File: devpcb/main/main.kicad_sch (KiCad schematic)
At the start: 17 parts, among them U1 DRV8301DCAR, U2 RP2040

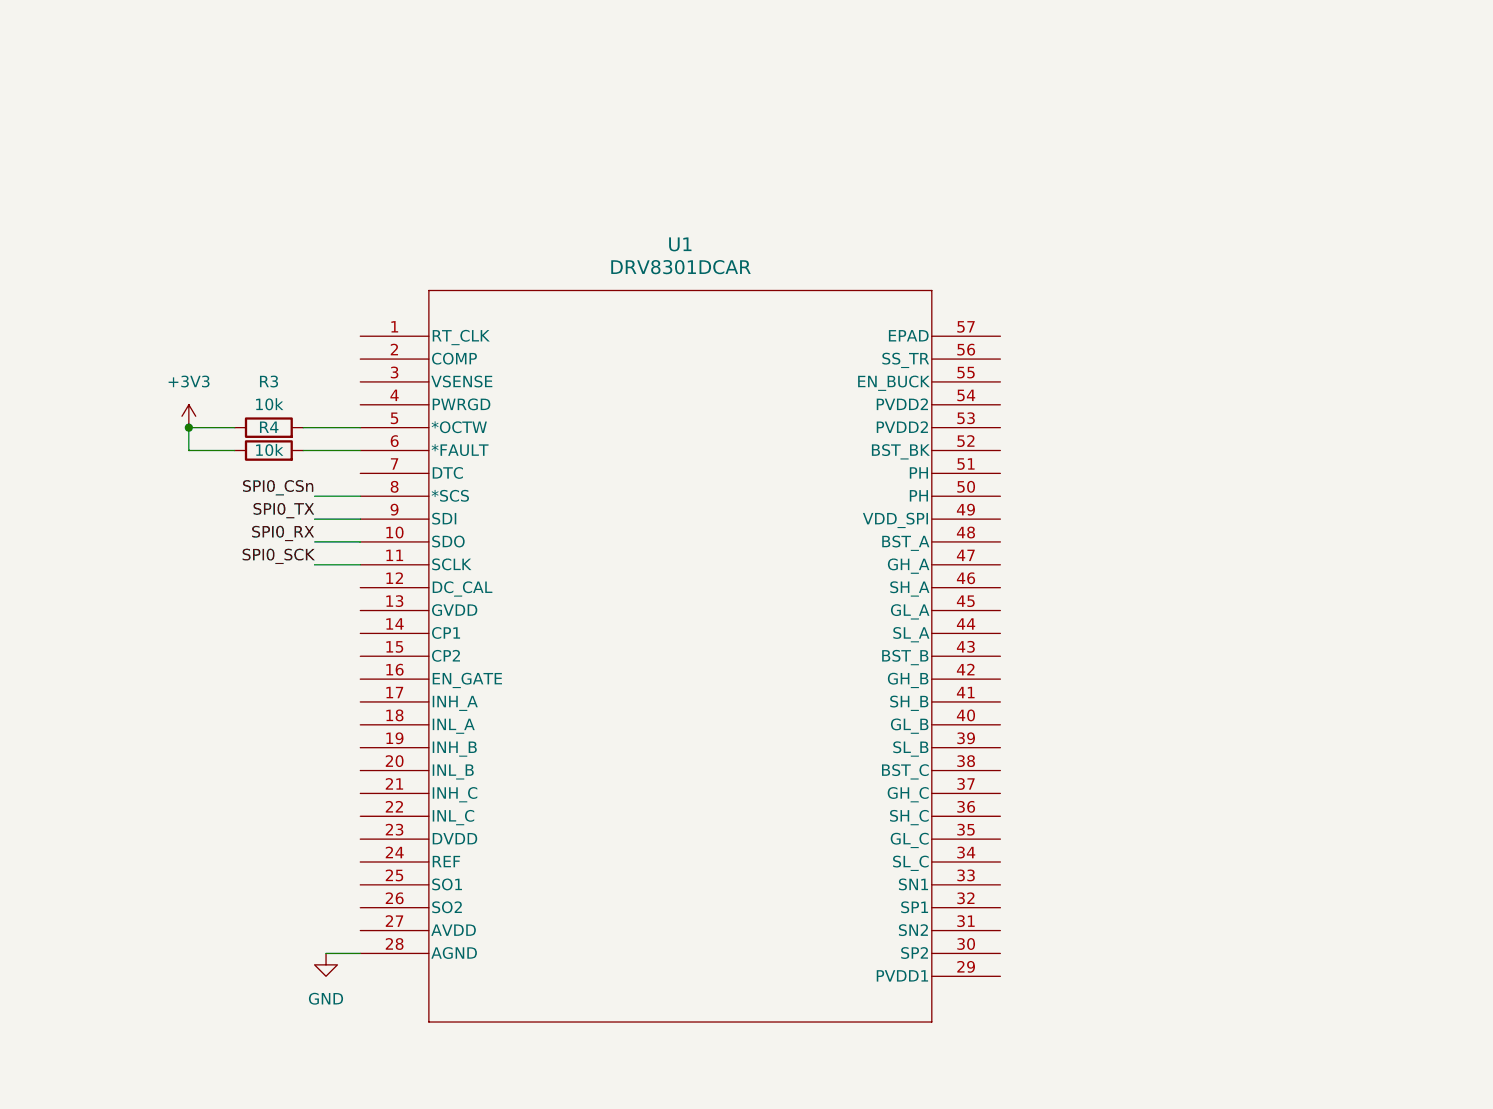
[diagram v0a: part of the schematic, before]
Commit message: gtg sep 19 5pm
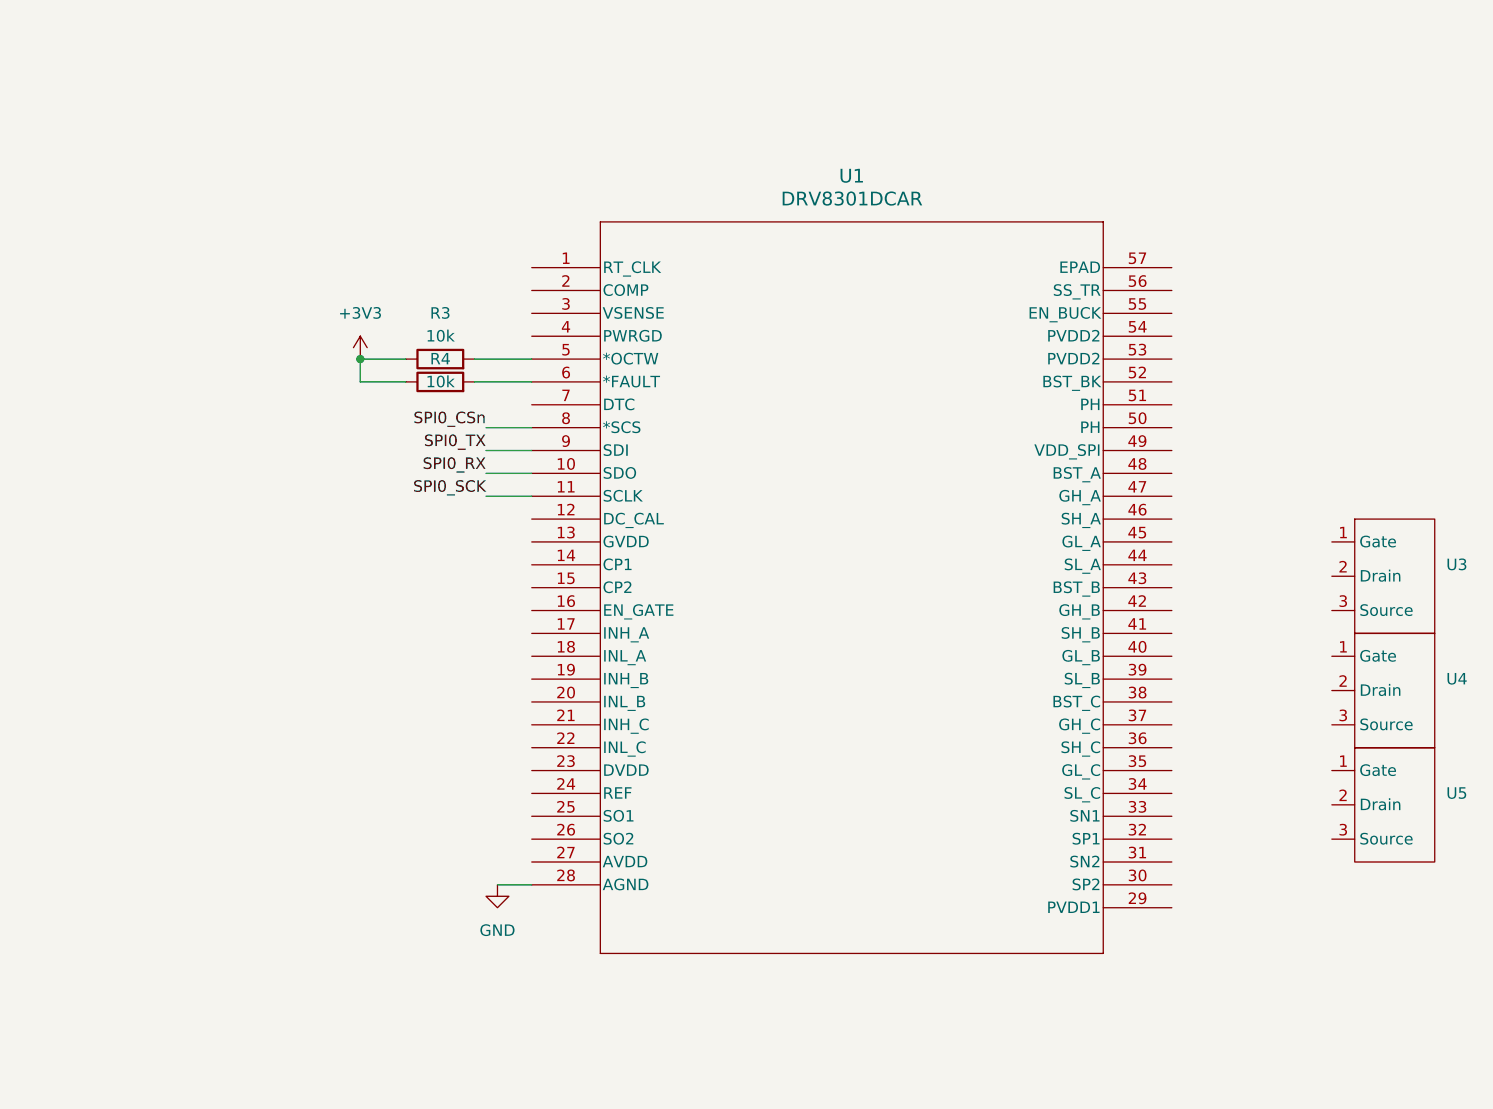
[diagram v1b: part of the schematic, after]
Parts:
- added U3, U4, U5: ~, Package_TO_SOT_THT:TO-220-3_Vertical, symbol RS100N135T:RS100N135T
- U1: footprint DCA56_6P35X3P61 -> DRV8301DCAR:DCA56_6P35X3P61
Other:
- moved on the sheet: R3, R4, U1

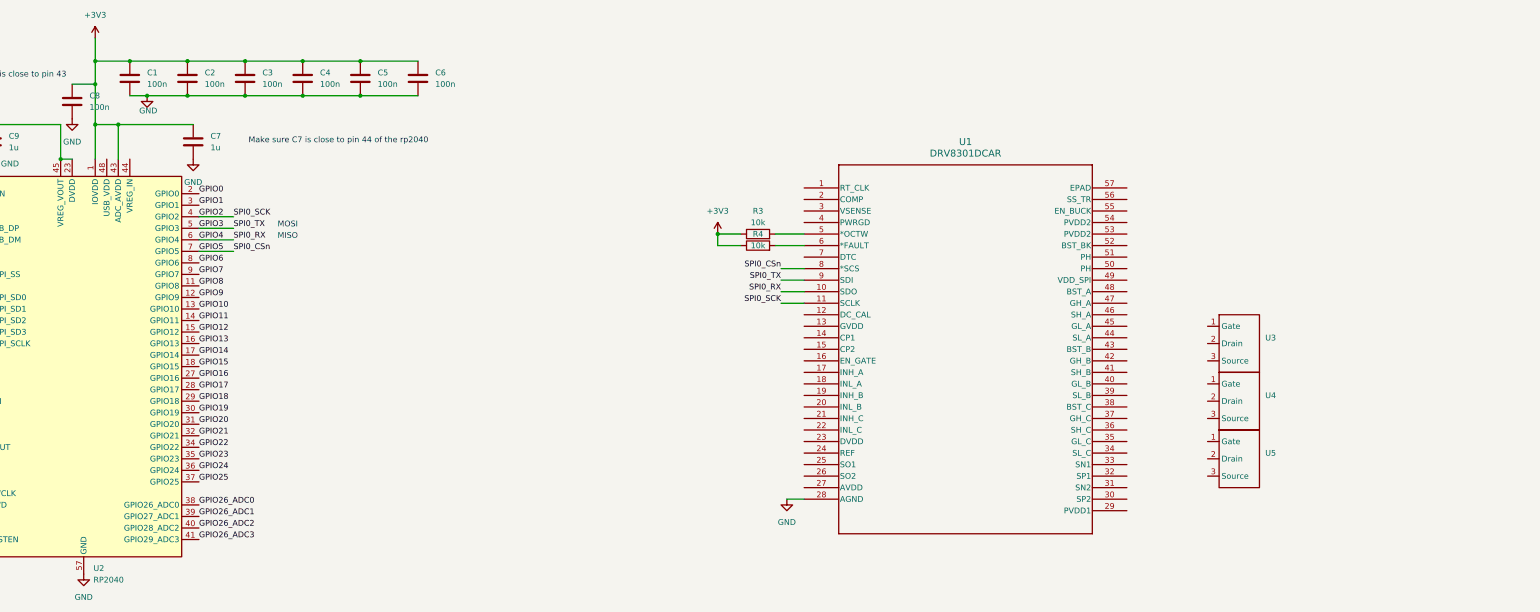
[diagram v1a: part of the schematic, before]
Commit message: a
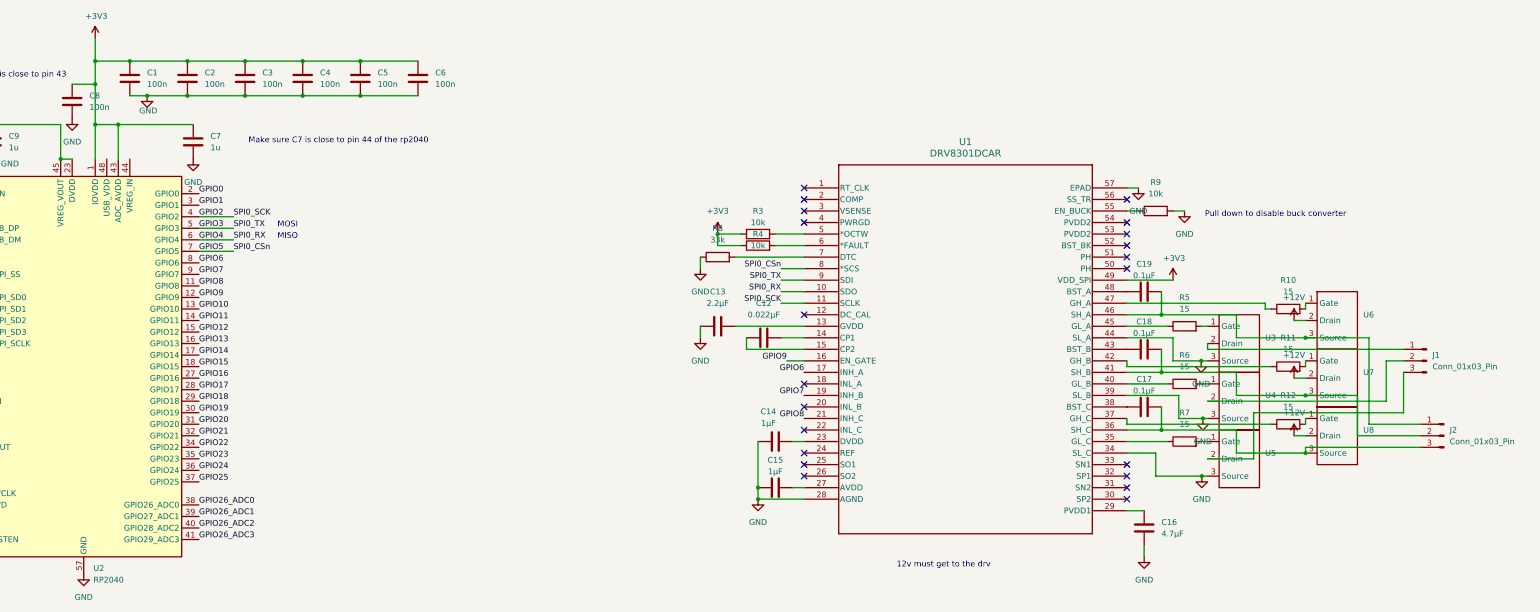
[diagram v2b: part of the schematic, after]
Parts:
- added C12: 0.022µF, Capacitor_SMD:C_0402_1005Metric_Pad0.74x0.62mm_HandSolder, symbol Device:C
- added C13: 2.2µF, Capacitor_SMD:C_0805_2012Metric, symbol Device:C
- added C14, C15: 1µF, Capacitor_SMD:C_0603_1608Metric, symbol Device:C
- added C16: 4.7µF, Capacitor_SMD:C_0805_2012Metric, symbol Device:C
- added C17, C18, C19: 0.1µF, Capacitor_SMD:C_0603_1608Metric, symbol Device:C
- added J1, J2: Conn_01x03_Pin, Connector_PinHeader_2.54mm:PinHeader_1x03_P2.54mm_Vertical, symbol Connector:Conn_01x03_Pin
- added R10, R11, R12, R5, R6, R7: 15, Resistor_SMD:R_0402_1005Metric, symbol Device:R
- added R8: 33k, Resistor_SMD:R_0402_1005Metric, symbol Device:R
- added R9: 10k, Resistor_SMD:R_0402_1005Metric, symbol Device:R
- added U6, U7, U8: ~, Package_TO_SOT_THT:TO-220-3_Vertical, symbol RS100N135T:RS100N135T
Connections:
- net +3V3: now also U1.49 (VDD_SPI)
- net GND: now also U1.34 (SL_C), U1.39 (SL_B), U1.44 (SL_A), U1.57 (EPAD), U3.3 (Source), U4.3 (Source), U5.3 (Source), C13.1, C14.1, C15.1, C16.2, R8.1, R9.2
- net GPIO6: now also U1.17 (INH_A)
- net GPIO7: now also U1.19 (INH_B)
- net GPIO8: now also U1.21 (INH_C)
- net GPIO9: now also U1.16 (EN_GATE)
- net at U5.1 (Gate): now also R7.2
- net at U5.2 (Drain): now also J1.3 (Pin_3)
- net at U3.1 (Gate): now also R5.2
- net at U3.2 (Drain): now also J1.1 (Pin_1)
- net at U4.1 (Gate): now also R6.2
- net at U4.2 (Drain): now also J1.2 (Pin_2)
- net at U1.13 (GVDD): now also C13.2
- net at U1.14 (CP1): now also C12.2
- net at U1.15 (CP2): now also C12.1
- net at U1.23 (DVDD): now also C14.2
- net at U1.27 (AVDD): now also C15.2
- net at U1.29 (PVDD1): now also C16.1
- net at U1.35 (GL_C): now also R7.1
- net at U1.36 (SH_C): now also C17.2, J2.3 (Pin_3), U8.3 (Source)
- net at U1.37 (GH_C): now also R12.1
- net at U1.38 (BST_C): now also C17.1
- net at U1.40 (GL_B): now also R6.1
- net at U1.41 (SH_B): now also C18.2, J2.2 (Pin_2), U7.3 (Source)
- net at U1.42 (GH_B): now also R11.1
- net at U1.43 (BST_B): now also C18.1
- net at U1.45 (GL_A): now also R5.1
- net at U1.46 (SH_A): now also C19.2, J2.1 (Pin_1), U6.3 (Source)
- net at U1.47 (GH_A): now also R10.1
- net at U1.48 (BST_A): now also C19.1
- net at U1.55 (EN_BUCK): now also R9.1
- net at U1.7 (DTC): now also R8.2
- new net: R10.2, U6.1 (Gate)
- new net: R11.2, U7.1 (Gate)
- new net: R12.2, U8.1 (Gate)
- new net +12V: U6.2 (Drain), U7.2 (Drain), U8.2 (Drain)
- no-connect marks 0 -> 21
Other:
- note added: "12v must get to the drv"
- note added: "Pull down to disable buck converter"
